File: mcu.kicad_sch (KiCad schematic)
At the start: 30 parts, among them Q1 2N7002, Q2 2N7002, Q3 2N7002, Q4 2N7002, Q5 2N7002, Q6 2N7002, U11 NUCLEOH723ZG

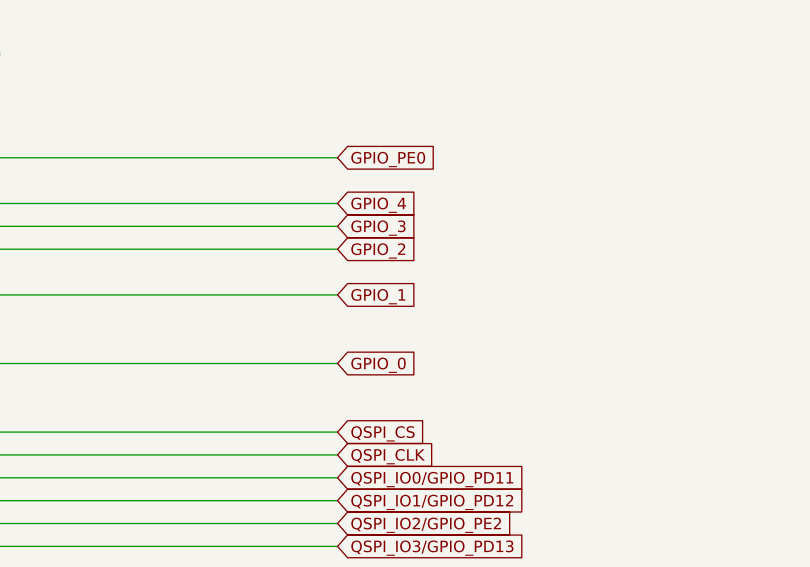
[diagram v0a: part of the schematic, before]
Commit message: Place all elements after rework
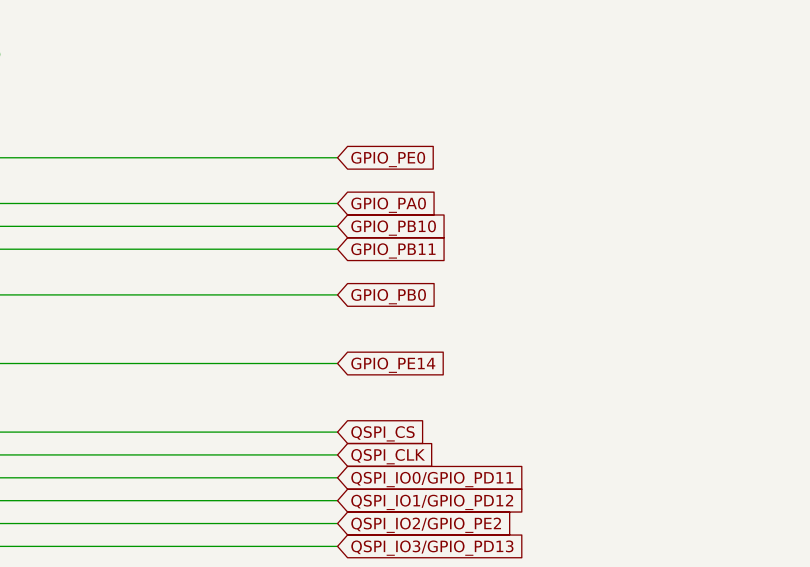
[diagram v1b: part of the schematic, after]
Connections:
- net GPIO_0 renamed GPIO_PE14
- net GPIO_1 renamed GPIO_PB0
- net GPIO_2 renamed GPIO_PB11
- net GPIO_3 renamed GPIO_PB10
- net GPIO_4 renamed GPIO_PA0
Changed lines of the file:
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@@
+	)
+	(no_connect
+		(at 308.61 158.75)
 	)
 	(no_connect
@@
 	(no_connect
 		(at 242.57 123.19)
-	)
-	(no_connect
-		(at 308.61 158.75)
 	)
 	(no_connect
@@
 		)
 	)
-	(global_label "GPIO_3"
+	(global_label "GPIO_PB10"
 		(shape input)
 		(at 350.52 190.5 0)
@@
 		)
 		(property "Intersheetrefs" "${INTERSHEET_REFS}"
-			(at 360.1576 190.5 0)
+			(at 363.9071 190.5 0)
 			(effects
 				(font
@@
 		)
 	)
-	(global_label "GPIO_0"
+	(global_label "GPIO_PE14"
 		(shape input)
 		(at 350.52 205.74 0)
@@
 		)
 		(property "Intersheetrefs" "${INTERSHEET_REFS}"
-			(at 360.1576 205.74 0)
+			(at 363.7861 205.74 0)
 			(effects
 				(font
@@
 		)
 	)
-	(global_label "GPIO_1"
+	(global_label "GPIO_PB0"
 		(shape input)
 		(at 350.52 198.12 0)
@@
 		)
 		(property "Intersheetrefs" "${INTERSHEET_REFS}"
-			(at 360.1576 198.12 0)
+			(at 362.6976 198.12 0)
 			(effects
 				(font
@@
 		)
 	)
-	(global_label "GPIO_4"
+	(global_label "GPIO_PA0"
 		(shape input)
 		(at 350.52 187.96 0)
@@
 		)
 		(property "Intersheetrefs" "${INTERSHEET_REFS}"
-			(at 360.1576 187.96 0)
+			(at 362.5162 187.96 0)
 			(effects
 				(font
@@
 		)
 	)
-	(global_label "GPIO_2"
+	(global_label "GPIO_PB11"
 		(shape input)
 		(at 350.52 193.04 0)
@@
 		)
 		(property "Intersheetrefs" "${INTERSHEET_REFS}"
-			(at 360.1576 193.04 0)
-			(effects
-				(font
+			(at 363.9071 193.04 0)
+			(effects
+				(font
